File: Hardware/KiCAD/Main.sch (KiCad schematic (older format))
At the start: 4 parts

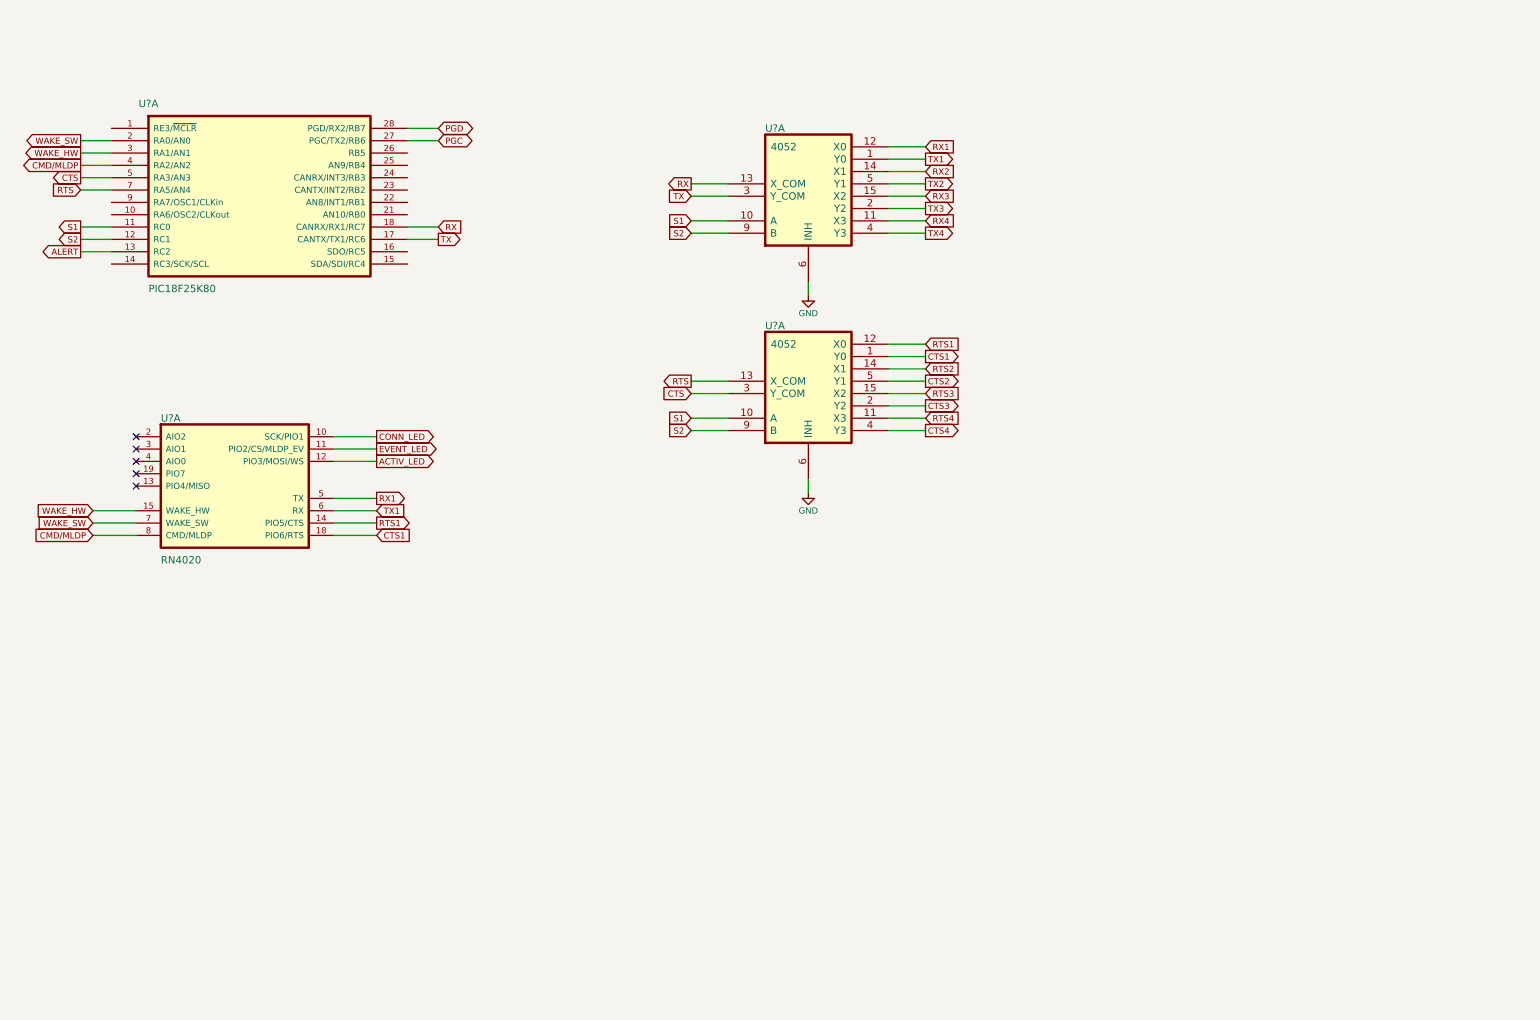
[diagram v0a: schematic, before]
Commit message: More work on the schematic
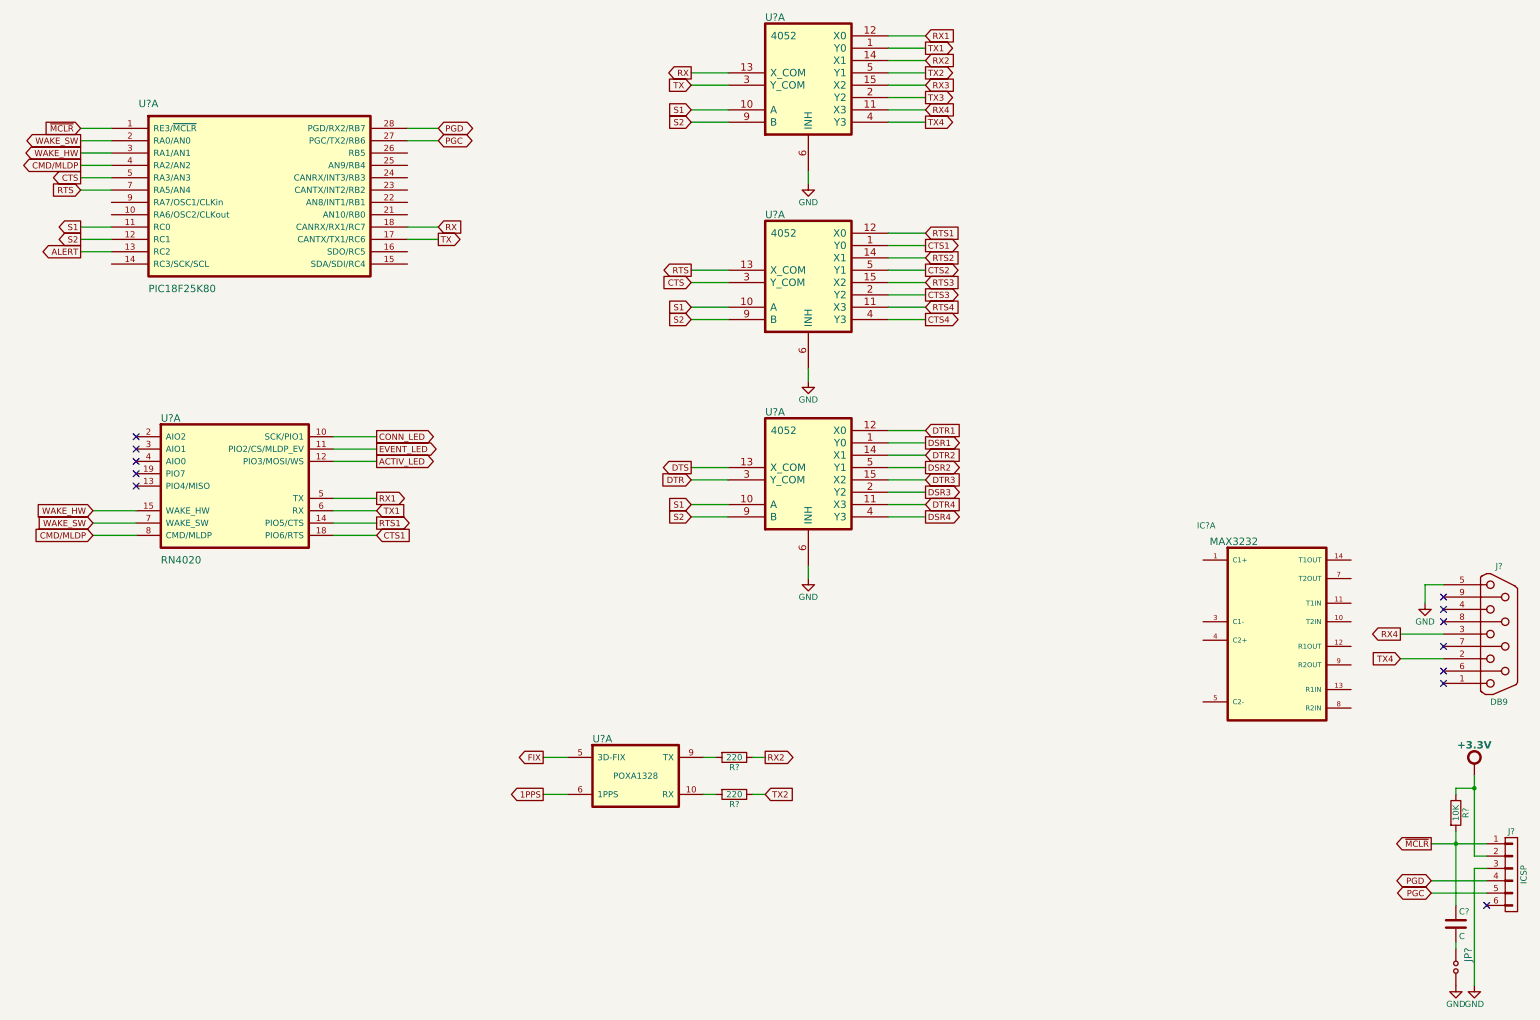
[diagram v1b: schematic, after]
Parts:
- added C?: C, symbol C
- added IC?: MAX3232_BJH, maxim-DIL16, symbol MAX3232_BJH
- added J?: ICSP, symbol CONN_01X06
- added J?: DB9, symbol DB9
- added JP?: Jumper, symbol Jumper
- added R?: 10K, symbol R
- added R? (x2): 220, symbol R
- added U?: POXA1328-007, symbol POXA1328-007
- added U?: 4000series-4052, DIP16, symbol 4000series-4052
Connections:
- net GND: now also J?.3 (P3), J?.5, JP?.2, U?.6 (INH)
- net PGC: now also J?.5 (P5)
- net PGD: now also J?.4 (P4)
- net RX2: now also R?.1
- net RX4: now also J?.3
- net S1: now also U?.10 (A)
- net S2: now also U?.9 (B)
- net TX2: now also R?.1
- net TX4: now also J?.2
- net ~MCLR: now reaches U?.1 (RE3/~MCLR)
- net ~MCLR: now also C?.1, J?.1 (P1), R?.2
- new net: C?.2, JP?.1
- new net: R?.2, U?.10 (RX)
- new net: R?.2, U?.9 (TX)
- new net +3.3V: J?.2 (P2), R?.1
- new net 1PPS: U?.6 (1PPS)
- new net DSR1: U?.1 (Y0)
- new net DSR2: U?.5 (Y1)
- new net DSR3: U?.2 (Y2)
- new net DSR4: U?.4 (Y3)
- new net DTR: U?.3 (Y_COM)
- new net DTR1: U?.12 (X0)
- new net DTR2: U?.14 (X1)
- new net DTR3: U?.15 (X2)
- new net DTR4: U?.11 (X3)
- new net DTS: U?.13 (X_COM)
- new net FIX: U?.5 (3D-FIX)
- no-connect marks 5 -> 12
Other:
- moved on the sheet: U?A
